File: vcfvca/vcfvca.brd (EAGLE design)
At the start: 160 x 50.5 mm, 104 parts, among them IC1 LM13700N, IC2 LM4558N, IC3 LM13700N, IC4 LM13700N, IC5 LM4558N, J1 POWER, J2 FREQ, J3 RES, J4 AMP, J5 AUD_IN, J6 AUD_OUT, Q1 BF245, Q10 2N3906, Q2 BF245, Q3 2N3906, Q4 BF245, Q5 BF245, Q6 2N3906, Q7 2N3906, Q8 2N3904, Q9 2N3906

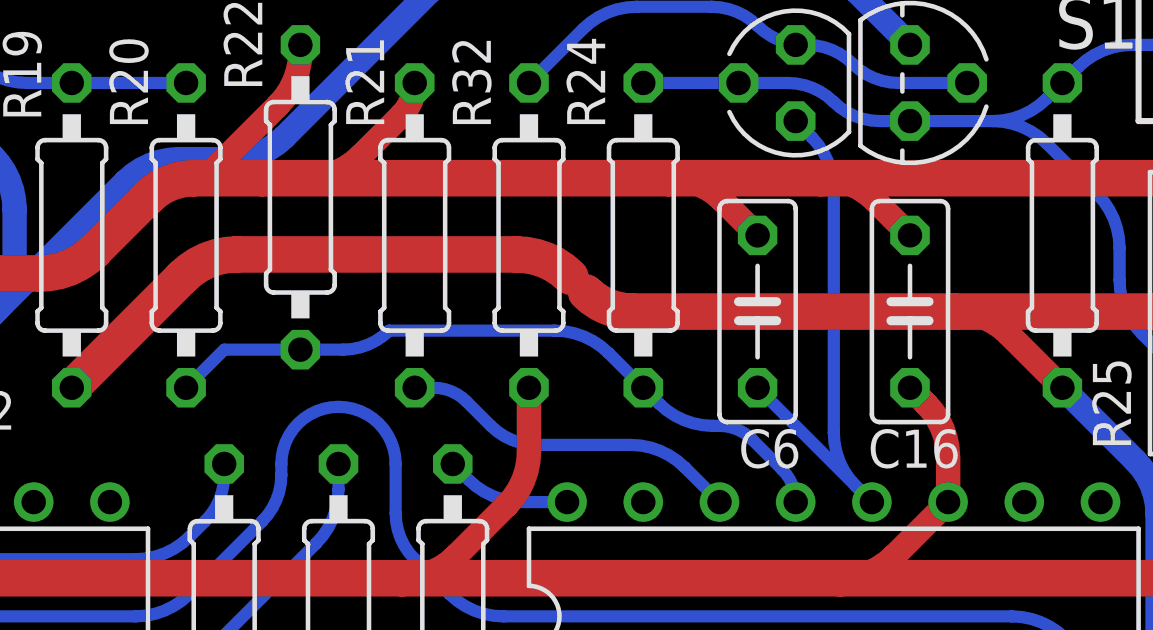
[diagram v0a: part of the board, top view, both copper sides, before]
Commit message: Minor fixes
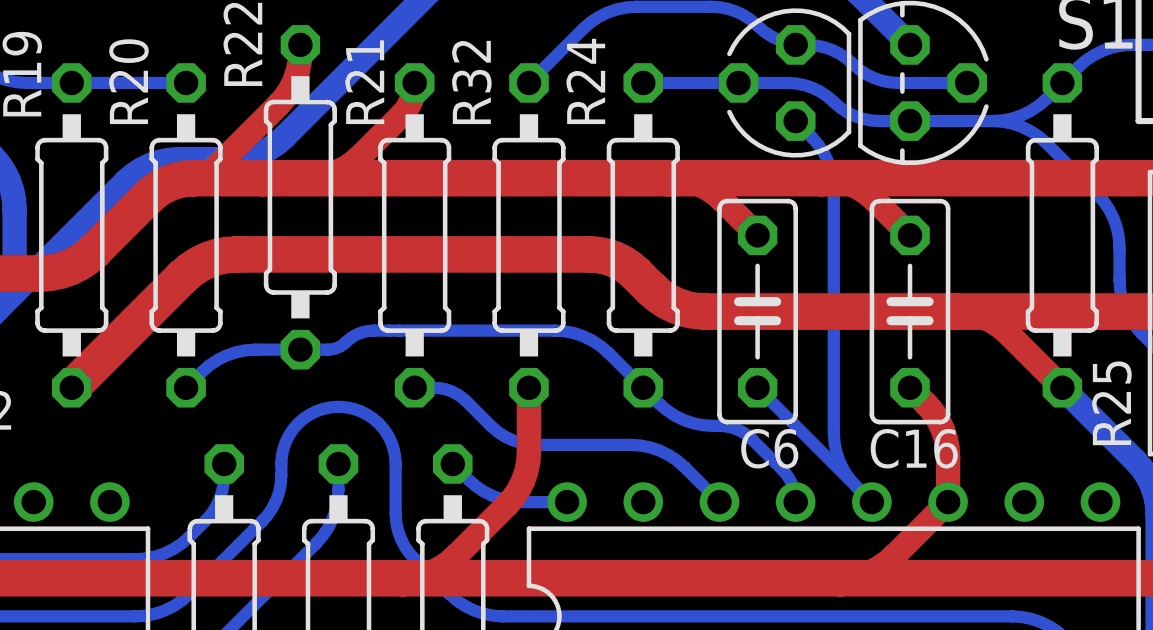
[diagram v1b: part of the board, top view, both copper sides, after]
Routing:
- net -15V: track 292.0 -> 288.4 mm
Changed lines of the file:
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@@
 <wire x1="20.583025" y1="25.4" x2="24.13" y2="25.4" width="0.8128" layer="1"/>
 <wire x1="74.82105" y1="37.99105" x2="76.617103125" y2="38.735" width="0.8128" layer="1" curve="-45"/>
-<wire x1="85.942896875" y1="38.735" x2="87.73895" y2="37.99105" width="0.8128" layer="1" curve="-45"/>
-<wire x1="87.73895" y1="37.99105" x2="88.265" y2="37.465" width="0.8128" layer="1"/>
-<wire x1="89.798025" y1="36.83" x2="88.265" y2="37.465" width="0.8128" layer="1" curve="-45"/>
 <wire x1="102.34395" y1="36.08605" x2="100.547896875" y2="36.83" width="0.8128" layer="1" curve="45"/>
 <wire x1="102.34395" y1="36.08605" x2="104.14" y2="34.29" width="0.8128" layer="1"/>
@@
 <wire x1="71.12" y1="34.29" x2="74.82105" y2="37.99105" width="1.2192" layer="1"/>
 <wire x1="74.82105" y1="37.99105" x2="76.617103125" y2="38.735" width="1.2192" layer="1" curve="-45"/>
-<wire x1="76.617103125" y1="38.735" x2="85.942896875" y2="38.735" width="1.2192" layer="1"/>
-<wire x1="85.942896875" y1="38.735" x2="87.73895" y2="37.99105" width="1.2192" layer="1" curve="-45"/>
-<wire x1="88.265" y1="37.465" x2="89.798025" y2="36.83" width="1.2192" layer="1" curve="45"/>
-<wire x1="89.798025" y1="36.83" x2="100.547896875" y2="36.83" width="1.2192" layer="1"/>
+<wire x1="76.617103125" y1="38.735" x2="88.382975" y2="38.735" width="1.2192" layer="1"/>
+<wire x1="92.238103125" y1="36.83" x2="100.547896875" y2="36.83" width="1.2192" layer="1"/>
 <wire x1="100.547896875" y1="36.83" x2="109.22" y2="36.83" width="1.2192" layer="1"/>
 <wire x1="11.049" y1="21.59" x2="11.049" y2="24.093896875" width="1.2192" layer="1"/>
@@
 <wire x1="10.30505" y1="25.88995" x2="10.16" y2="26.035" width="1.2192" layer="1"/>
 <wire x1="9.86255" y1="26.33245" x2="8.066496875" y2="27.0764" width="1.2192" layer="1" curve="45"/>
+<wire x1="88.382975" y1="38.735" x2="89.916" y2="38.1" width="1.2192" layer="1" curve="-45"/>
+<wire x1="89.916" y1="38.1" x2="90.44205" y2="37.57395" width="1.2192" layer="1"/>
+<wire x1="90.44205" y1="37.57395" x2="92.238103125" y2="36.83" width="1.2192" layer="1" curve="45"/>
 </signal>
 <signal name="N$2">
@@
 <contactref element="R24" pad="1"/>
 <contactref element="IC3" pad="13"/>
-<wire x1="78.74" y1="35.56" x2="76.2" y2="35.56" width="0.4064" layer="16"/>
-<wire x1="74.93" y1="34.29" x2="76.2" y2="35.56" width="0.4064" layer="16"/>
-<wire x1="78.74" y1="35.56" x2="80.164078125" y2="35.56" width="0.4064" layer="16"/>
-<wire x1="80.164078125" y1="35.56" x2="81.697103125" y2="36.195" width="0.4064" layer="16" curve="45"/>
 <wire x1="95.25" y1="30.48" x2="94.8009875" y2="31.5640125" width="0.4064" layer="16" curve="45"/>
 <wire x1="93.7940125" y1="32.5709875" x2="92.71" y2="33.02" width="0.4064" layer="16" curve="45"/>
@@
 <wire x1="90.17" y1="34.29" x2="89.00895" y2="35.45105" width="0.4064" layer="16"/>
 <wire x1="89.00895" y1="35.45105" x2="87.212896875" y2="36.195" width="0.4064" layer="16" curve="45"/>
-<wire x1="87.212896875" y1="36.195" x2="81.697103125" y2="36.195" width="0.4064" layer="16"/>
+<wire x1="87.212896875" y1="36.195" x2="82.042" y2="36.195" width="0.4064" layer="16"/>
+<wire x1="82.042" y1="36.195" x2="81.697103125" y2="36.195" width="0.4064" layer="16"/>
+<wire x1="74.93" y1="34.29" x2="75.45605" y2="34.81605" width="0.4064" layer="16"/>
+<wire x1="75.45605" y1="34.81605" x2="77.252103125" y2="35.56" width="0.4064" layer="16" curve="-45"/>
+<wire x1="77.252103125" y1="35.56" x2="78.74" y2="35.56" width="0.4064" layer="16"/>
+<wire x1="78.74" y1="35.56" x2="79.650790625" y2="35.56" width="0.4064" layer="16"/>
+<wire x1="79.650790625" y1="35.56" x2="80.264" y2="35.814" width="0.4064" layer="16" curve="45"/>
+<wire x1="80.264" y1="35.814" x2="81.183815625" y2="36.195" width="0.4064" layer="16" curve="-45"/>
+<wire x1="81.183815625" y1="36.195" x2="81.697103125" y2="36.195" width="0.4064" layer="16"/>
 </signal>
 <signal name="N$21">
